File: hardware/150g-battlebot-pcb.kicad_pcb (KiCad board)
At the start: 4 copper layers, 65 x 69 mm, 93 parts, among them J401 Conn_ST_STDC14, M201 M1_CONN, M202 M2_CONN, M203 M3_CONN, M204 M4_CONN, U103 A7105, U301 MIC5504-3.3YM5, U401 STM32G431C6Ux, U501 LIS3DH, U601 STSPIN240, U602 STSPIN240, Y201 16_mhz, Y401 16_mhz, Y402 Q13FC1350000400

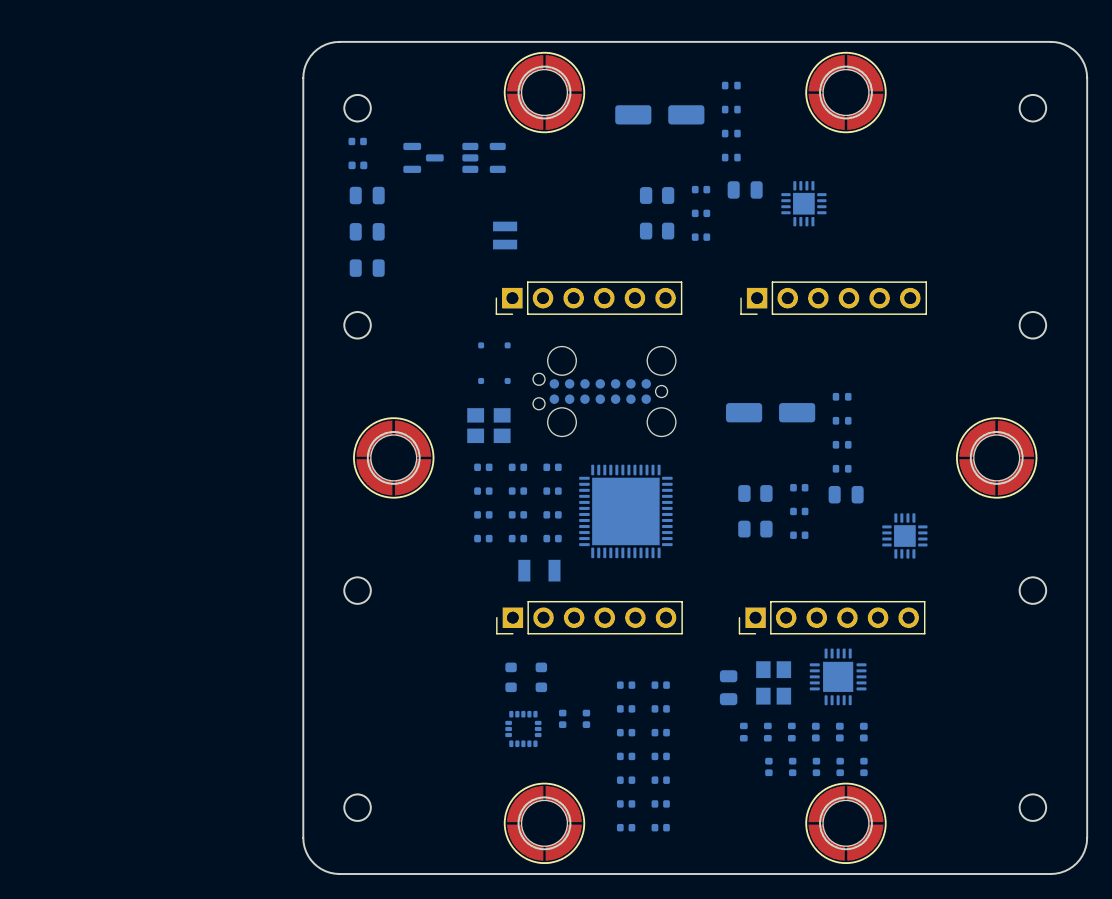
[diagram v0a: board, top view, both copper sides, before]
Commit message: asdf
Signed-off-by: Connor Rigby <connorr@hey.com>
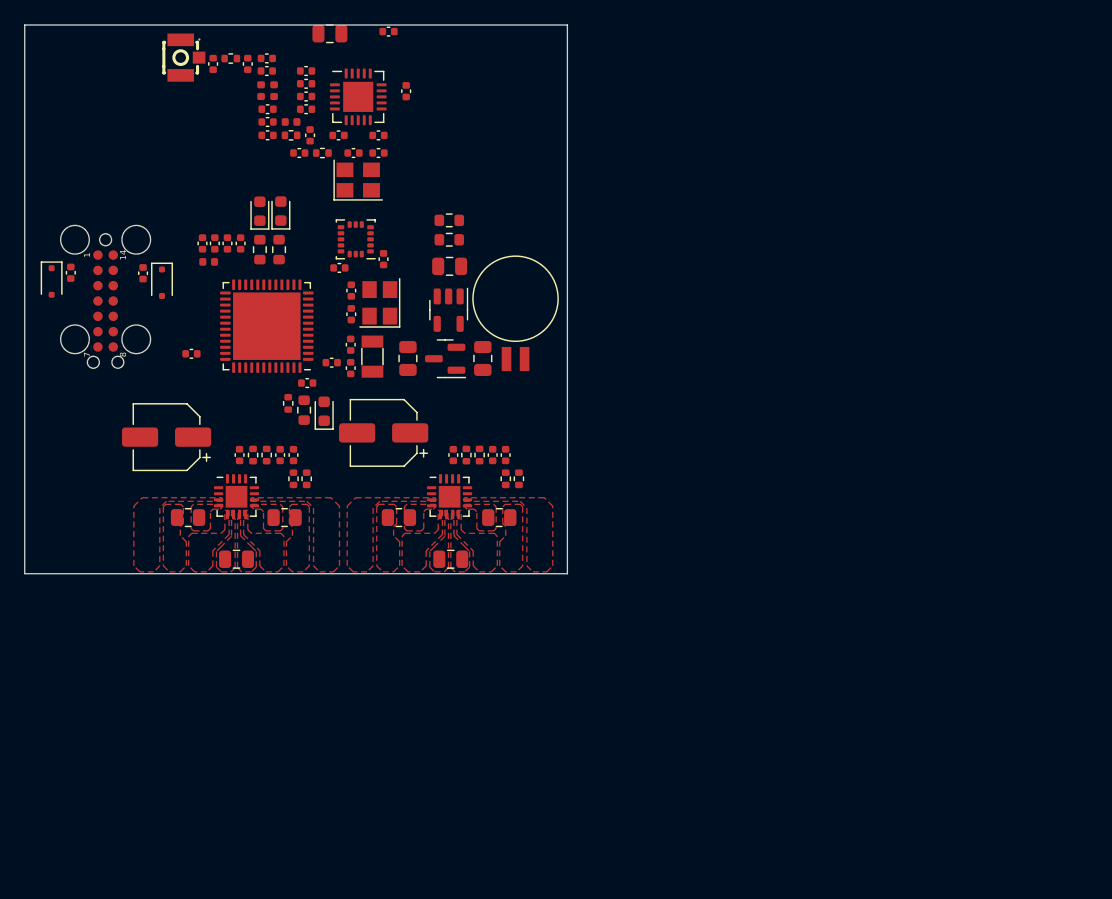
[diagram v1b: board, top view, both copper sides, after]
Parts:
- removed M201: M1_CONN, Connector_PinHeader_2.54mm:PinHeader_1x06_P2.54mm_Vertical
- removed M202: M2_CONN, Connector_PinHeader_2.54mm:PinHeader_1x06_P2.54mm_Vertical
- removed M203: M3_CONN, Connector_PinHeader_2.54mm:PinHeader_1x06_P2.54mm_Vertical
- removed M204: M4_CONN, Connector_PinHeader_2.54mm:PinHeader_1x06_P2.54mm_Vertical
- removed REF** (x6): SMD_BD5.6-L5.6-W5.6-D3.6, LCSC_Connector:SMD_BD5.6-L5.6-W5.6-D3.6
- added AE201: Antenna_Chip, LCSC_Antenna:IPEX-SMD_BWIPX-1-001E, F.Cu at (37.4, 26.8)
- added D403: LED_0603_DNP, LED_SMD:LED_0603_1608Metric, F.Cu at (49.2, 56.1)
- added D404: LED_0603_DNP, LED_SMD:LED_0603_1608Metric, F.Cu at (45.6, 39.5)
- added D405: LED_0603_DNP, LED_SMD:LED_0603_1608Metric, F.Cu at (43.9, 39.5)
- added R401: R_0402_1k, Resistor_SMD:R_0402_1005Metric, F.Cu at (46.2, 55.5)
- added R402: R_0603_DNP, Resistor_SMD:R_0603_1608Metric, F.Cu at (47.6, 56.0)
- added R403: R_0603_DNP, Resistor_SMD:R_0603_1608Metric, F.Cu at (45.5, 42.7)
- added R404: R_0603_DNP, Resistor_SMD:R_0603_1608Metric, F.Cu at (43.9, 42.7)
- BT302, C201, C202, C203, C204, C205, C206, C207, C208, C209, C210, C211, C212, C213, C214, C215, C216, C217, C218, C219, C220, C301, C302, C303, C304, C401, C402, C403, C404, C405, C406, C407, C408, C409, C410, C411, C412, C501, C502, C601, C602, C603, C604, C605, C606, C607, C608, C609, C610, D301, D401, D402, FB301, J401, L202, L203, L204, R201, R202, R203, R501, R502, R601, R602, R603, R604, R605, R606, R607, R608, R609, R610, R611, R612, U103, U301, U401, U501, U601, U602, Y201, Y401, Y402: moved to F.Cu
- moved C217 75.6 mm to (44.5, 26.9), turned to 0 degrees
- moved C219 75.5 mm to (40.0, 27.3)
- moved C216 73.6 mm to (44.5, 31.1), turned to 180 degrees
- moved C218 73.5 mm to (44.5, 27.9), turned to 0 degrees
- moved C220 72.6 mm to (42.9, 27.3)
- moved L202 72.3 mm to (45.1, 29.5), turned to -90 degrees
- moved L204 70.3 mm to (44.0, 29.5), turned to -90 degrees
- moved R203 70.2 mm to (41.5, 26.9), turned to 180 degrees
- moved C202 68.9 mm to (54.6, 24.6)
- moved L203 68.0 mm to (46.5, 32.1), turned to 180 degrees
- moved C210 65.6 mm to (47.7, 30.0)
- moved R201 64.6 mm to (46.5, 33.2), turned to 0 degrees
- moved C211 63.6 mm to (44.5, 32.1)
- moved C201 63.5 mm to (49.7, 24.8), turned to 180 degrees
- moved C209 63.3 mm to (50.4, 33.3)
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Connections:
- BT302 pad 1: +BATT -> Net-(BT302-+)
- C303 pad 1: Net-(C303-Pad1) -> +BATT
- C501 pad 1: Net-(U501-VDD) -> VDD
- C502 pad 1: Net-(U501-VDD) -> VDD
- C601 pad 1: /MotorDrivers/~{RESET} -> /Application/~{RESET}
- C602 pad 1: /MotorDrivers/EN_FAULT -> /Application/FAULT
- C608 pad 1: /MotorDrivers/~{RESET} -> /Application/FAULT
- C610 pad 1: /MotorDrivers/~{RESET} -> /Application/~{RESET}
- D301 pad 1: +BATT -> Net-(BT302-+)
- D301 pad 3: Net-(C303-Pad1) -> +BATT
- FB301 pad 1: Net-(C303-Pad1) -> VDD
- R501 pad 1: /Sensors/VBAT_SENSE -> /Application/BAT_SENSE
- R502 pad 2: /Sensors/VBAT_SENSE -> /Application/BAT_SENSE
- R601 pad 2: /MotorDrivers/~{RESET} -> /Application/~{RESET}
- R604 pad 2: /MotorDrivers/EN_FAULT -> /Application/FAULT
- R608 pad 2: /MotorDrivers/~{RESET} -> /Application/FAULT
- R612 pad 2: /MotorDrivers/~{RESET} -> /Application/~{RESET}
- U103 pad 11: /RF/SCS -> /Application/~{RF_CS}
- U103 pad 12: /RF/SCK -> /Application/SPI1_SCK
- U103 pad 14: /RF/SDIO -> /Application/SPI1_MOSI
- U103 pad 16: /RF/GIO1 -> /Application/SPI1_MISO
- U103 pad 17: /RF/GIO2 -> /Application/RF_GIO2
- U401 pad 10: unconnected-(U401-PA2-Pad10) -> /Application/IMU_INT1
- U401 pad 11: unconnected-(U401-PA3-Pad11) -> /Application/IMU_INT2
- U401 pad 12: unconnected-(U401-PA4-Pad12) -> /Application/~{IMU_CS}
- U401 pad 13: unconnected-(U401-PA5-Pad13) -> /Application/SPI1_SCK
- U401 pad 14: unconnected-(U401-PA6-Pad14) -> /Application/SPI1_MISO
- U401 pad 15: unconnected-(U401-PA7-Pad15) -> /Application/SPI1_MOSI
- U401 pad 16: unconnected-(U401-PC4-Pad16) -> /Application/~{RF_CS}
- U401 pad 17: unconnected-(U401-PB0-Pad17) -> /Application/RF_GIO2
- U401 pad 18: unconnected-(U401-PB1-Pad18) -> /Application/STATUS2
- U401 pad 19: unconnected-(U401-PB2-Pad19) -> /Application/STATUS3
- U401 pad 2: unconnected-(U401-PC13-Pad2) -> /Application/FAULT
- U401 pad 22: unconnected-(U401-PB10-Pad22) -> /Application/VCP_TX
- U401 pad 24: unconnected-(U401-PB11-Pad24) -> /Application/VCP_RX
- U401 pad 25: unconnected-(U401-PB12-Pad25) -> /Application/M2_DIR
- U401 pad 26: unconnected-(U401-PB13-Pad26) -> /Application/M1_DIR
- U401 pad 27: unconnected-(U401-PB14-Pad27) -> /Application/M3_PWM
- U401 pad 28: unconnected-(U401-PB15-Pad28) -> /Application/M4_PWM
- U401 pad 29: unconnected-(U401-PC6-Pad29) -> /Application/REF
- U401 pad 30: unconnected-(U401-PA8-Pad30) -> /Application/M1_ENCB
- U401 pad 31: unconnected-(U401-PA9-Pad31) -> /Application/M1_ENCA
- U401 pad 32: unconnected-(U401-PA10-Pad32) -> /Application/M1_PWM
- U401 pad 33: unconnected-(U401-PA11-Pad33) -> /Application/M2_PWM
- U401 pad 34: unconnected-(U401-PA12-Pad34) -> /Application/M4_ENCB
- U401 pad 36: unconnected-(U401-PA13-Pad36) -> /Application/JTMS
- U401 pad 37: unconnected-(U401-PA14-Pad37) -> /Application/JTCK
- U401 pad 38: unconnected-(U401-PA15-Pad38) -> /Application/JTDI
- U401 pad 39: unconnected-(U401-PC10-Pad39) -> /Application/M3_DIR
- U401 pad 40: unconnected-(U401-PC11-Pad40) -> /Application/M4_DIR
- U401 pad 41: unconnected-(U401-PB3-Pad41) -> /Application/JTDO
- U401 pad 42: unconnected-(U401-PB4-Pad42) -> /Application/M3_ENCA
- U401 pad 43: unconnected-(U401-PB5-Pad43) -> /Application/M3_ENCB
- U401 pad 44: unconnected-(U401-PB6-Pad44) -> /Application/M4_ENCA
- U401 pad 45: unconnected-(U401-PB7-Pad45) -> /Application/BAT_SENSE
- U401 pad 46: unconnected-(U401-PB8-Pad46) -> /Application/BOOT0
- U401 pad 47: unconnected-(U401-PB9-Pad47) -> /Application/STATUS1
- U401 pad 7: /Application/~{NRESET} -> /Application/~{RESET}
- U401 pad 8: unconnected-(U401-PA0-Pad8) -> /Application/M2_ENCA
- U401 pad 9: unconnected-(U401-PA1-Pad9) -> /Application/M2_ENCB
- U501 pad 1: Net-(U501-VDD) -> VDD
- U501 pad 11: /Sensors/INT1 -> /Application/IMU_INT1
- U501 pad 14: Net-(U501-VDD) -> VDD
- U501 pad 4: /Sensors/SCLK -> /Application/SPI1_SCK
- U501 pad 6: /Sensors/MOSI -> /Application/SPI1_MOSI
- U501 pad 7: /Sensors/MISO -> /Application/SPI1_MISO
- U501 pad 8: /Sensors/~{CS} -> /Application/~{IMU_CS}
- U501 pad 9: /Sensors/INT2 -> /Application/IMU_INT2
- U601 pad 1: /MotorDrivers/M1_PH -> /Application/M1_PWM
- U601 pad 11: /MotorDrivers/REF -> /Application/REF
- U601 pad 13: /MotorDrivers/EN_FAULT -> /Application/FAULT
- U601 pad 14: /MotorDrivers/~{RESET} -> /Application/~{RESET}
- U601 pad 15: /MotorDrivers/M2_PH -> /Application/M2_DIR
- U601 pad 16: /MotorDrivers/M2_PWM -> /Application/M2_PWM
- U601 pad 2: /MotorDrivers/M1_PWM -> /Application/M1_DIR
- U602 pad 1: /MotorDrivers/M3_PH -> /Application/M3_DIR
- U602 pad 11: /MotorDrivers/REF -> /Application/REF
- U602 pad 13: /MotorDrivers/~{RESET} -> /Application/FAULT
- U602 pad 14: /MotorDrivers/~{RESET} -> /Application/~{RESET}
- U602 pad 15: /MotorDrivers/M4_PH -> /Application/M4_DIR
- U602 pad 16: /MotorDrivers/M4_PWM -> /Application/M4_PWM
- U602 pad 2: /MotorDrivers/M3_PWM -> /Application/M3_PWM
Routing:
- added copper zone on F.Cu, net /MotorDrivers/M1_OUTA
- added copper zone on F.Cu, net /MotorDrivers/M1_OUTB
- added copper zone on F.Cu, net /MotorDrivers/M1_SENSE
- added copper zone on F.Cu, net /MotorDrivers/M2_OUTA
- added copper zone on F.Cu, net /MotorDrivers/M2_OUTB
- added copper zone on F.Cu, net /MotorDrivers/M2_SENSE
- added copper zone on F.Cu, net /MotorDrivers/M3_OUTA
- added copper zone on F.Cu, net /MotorDrivers/M3_OUTB
- added copper zone on F.Cu, net /MotorDrivers/M3_SENSE
- added copper zone on F.Cu, net /MotorDrivers/M4_OUTA
- added copper zone on F.Cu, net /MotorDrivers/M4_OUTB
- added copper zone on F.Cu, net /MotorDrivers/M4_SENSE
- added copper zone on F.Cu, net GND
- added copper zone on F.Cu, net VS
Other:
- board size 65 x 69 mm -> 45 x 45.5 mm
